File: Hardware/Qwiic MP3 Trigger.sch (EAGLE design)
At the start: 55 parts, among them J1 MICRO-SD, J3 PTH, J7 ISP, J8 3.5mm Audio, J9 Poke-Home, U1 TPA2005D1, U2 WT2003S, U3 AP2112-3.3V, U4 ATTINY84-ARDUINO

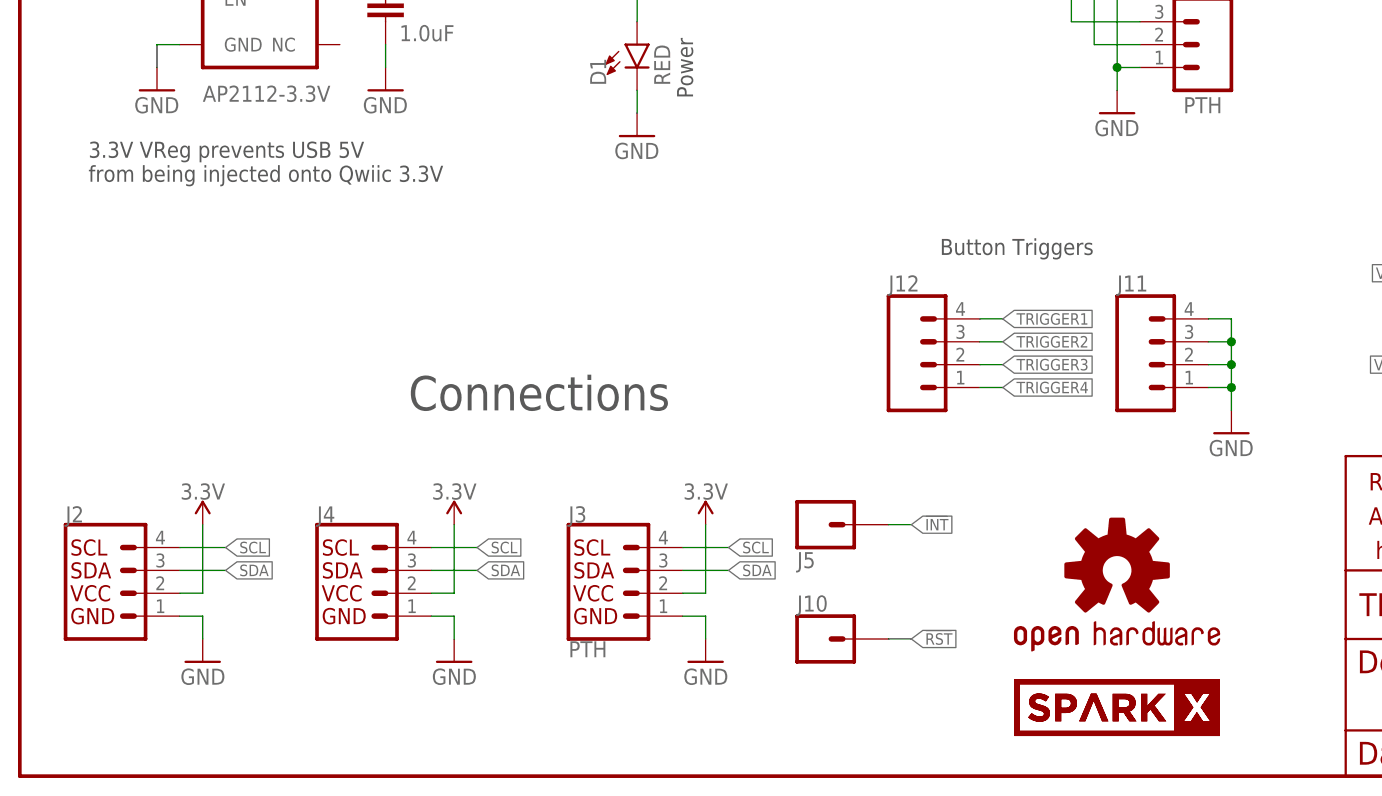
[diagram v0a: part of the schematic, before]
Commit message: File name clean up.
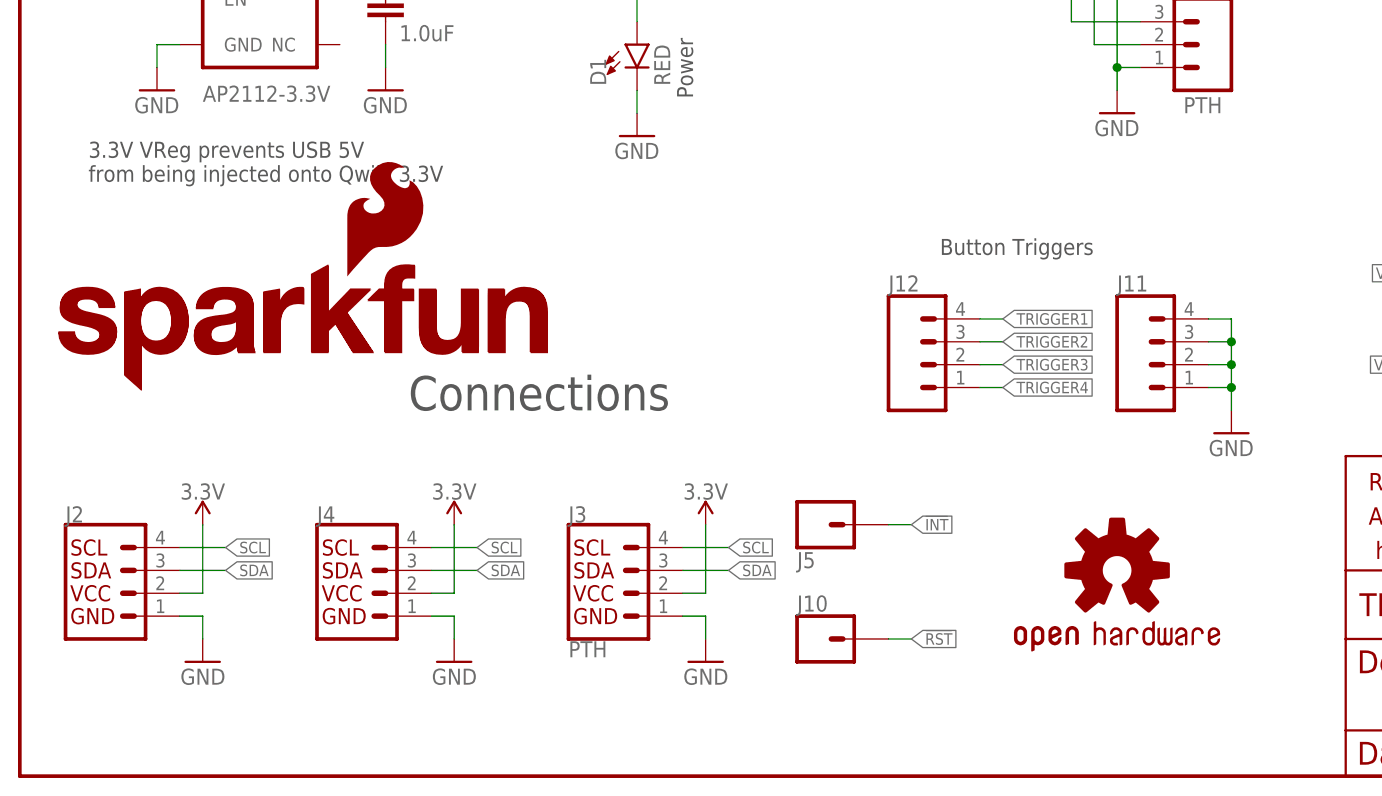
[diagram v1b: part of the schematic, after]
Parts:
- removed U$1: SPARKX-LOGO3, SparkX:SPARKX-LOGO3
- removed U$2: SPARKX-LOGO4, SparkX:SPARKX-LOGO4
- added LOGO2: SFE_LOGO_NAME.1_INCH, SparkFun-Aesthetics:SFE_LOGO_NAME.1_INCH
- added LOGO3: SFE_LOGO_NAME_FLAME.1_INCH, SparkFun-Aesthetics:SFE_LOGO_NAME_FLAME.1_INCH
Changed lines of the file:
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@@
 <class number="0" name="default" width="0" drill="0">
 </class>
-<class number="1" name="3.3V" width="0.1524" drill="0">
+<class number="1" name="3.3V" width="0.3048" drill="0">
 </class>
 </classes>
@@
 <part name="GND7" library="SparkFun-PowerSymbols" deviceset="GND" device=""/>
 <part name="FRAME1" library="SparkFun-Aesthetics" deviceset="FRAME-LETTER" device=""/>
-<part name="U$2" library="SparkX" deviceset="SPARKX-LOGO" device="4"/>
 <part name="SUPPLY8" library="SparkFun-PowerSymbols" deviceset="3.3V" device=""/>
 <part name="J4" library="SparkFun-Connectors" deviceset="QWIIC_CONNECTOR" device="JS-1MM"/>
 <part name="GND8" library="SparkFun-PowerSymbols" deviceset="GND" device=""/>
 <part name="LOGO1" library="SparkFun-Aesthetics" deviceset="OSHW-LOGO" device="MINI"/>
-<part name="U$1" library="SparkX" deviceset="SPARKX-LOGO" device="3" value="SPARKX-LOGO3"/>
 <part name="J5" library="SparkFun-Connectors" deviceset="CONN_01" device="PTH_NO_SILK_YES_STOP"/>
 <part name="JP1" library="SparkFun" deviceset="FIDUCIAL" device="UFIDUCIAL"/>
@@
 <part name="GND19" library="SparkFun-PowerSymbols" deviceset="GND" device=""/>
 <part name="GND20" library="SparkFun-PowerSymbols" deviceset="GND" device=""/>
+<part name="LOGO2" library="SparkFun-Aesthetics" deviceset="SFE_LOGO_NAME" device=".1_INCH"/>
+<part name="LOGO3" library="SparkFun-Aesthetics" deviceset="SFE_LOGO_NAME_FLAME" device=".1_INCH"/>
 </parts>
 <sheets>
@@
 <attribute name="DRAWING_NAME" x="162.814" y="17.78" size="2.7432" layer="94" font="vector"/>
 </instance>
-<instance part="U$2" gate="G$1" x="121.92" y="7.62" smashed="yes"/>
 <instance part="SUPPLY8" gate="G$1" x="48.26" y="27.94" smashed="yes" rot="MR0">
 <attribute name="VALUE" x="48.26" y="30.734" size="1.778" layer="96" rot="MR0" align="bottom-center"/>
@@
 </instance>
 <instance part="LOGO1" gate="G$1" x="121.92" y="22.86" smashed="yes"/>
-<instance part="U$1" gate="G$1" x="121.92" y="7.62" smashed="yes"/>
 <instance part="J5" gate="G$1" x="88.9" y="27.94" smashed="yes" rot="MR180">
 <attribute name="VALUE" x="86.36" y="32.766" size="1.778" layer="96" font="vector" rot="MR180"/>
@@
 <attribute name="VALUE" x="88.9" y="106.68" size="1.778" layer="96"/>
 </instance>
+<instance part="LOGO2" gate="G$1" x="2.286" y="42.926" smashed="yes"/>
+<instance part="LOGO3" gate="G$1" x="3.556" y="42.418" smashed="yes"/>
 </instances>
 <busses>
 </busses>
 <nets>
-<net name="3.3V" class="0">
+<net name="3.3V" class="1">
 <segment>
 <pinref part="J2" gate="G$1" pin="2"/>
